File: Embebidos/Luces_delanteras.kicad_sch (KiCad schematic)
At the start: 14 parts, among them J3 Pantallas I2C, J4 Luz_delantera, J5 Joystick, J6 RJ45, J7 RJ45, Q3 BSS138, Q4 DMP3056LSDQ-13

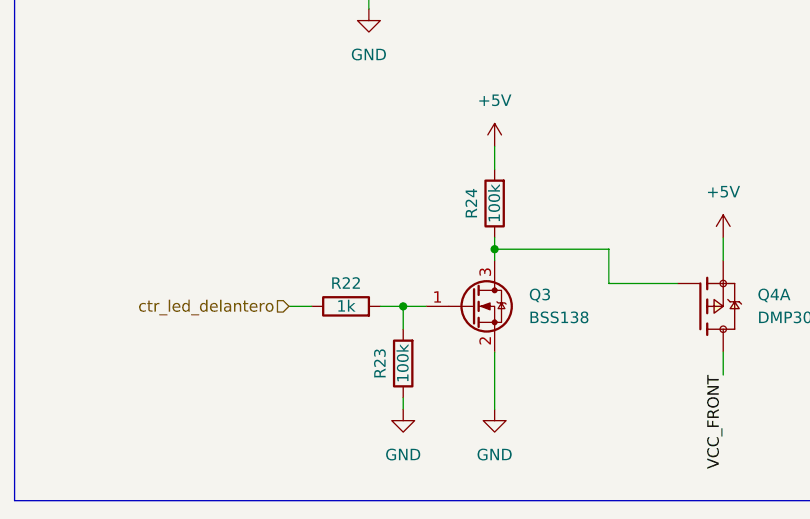
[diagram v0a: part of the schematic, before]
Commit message: nosex2
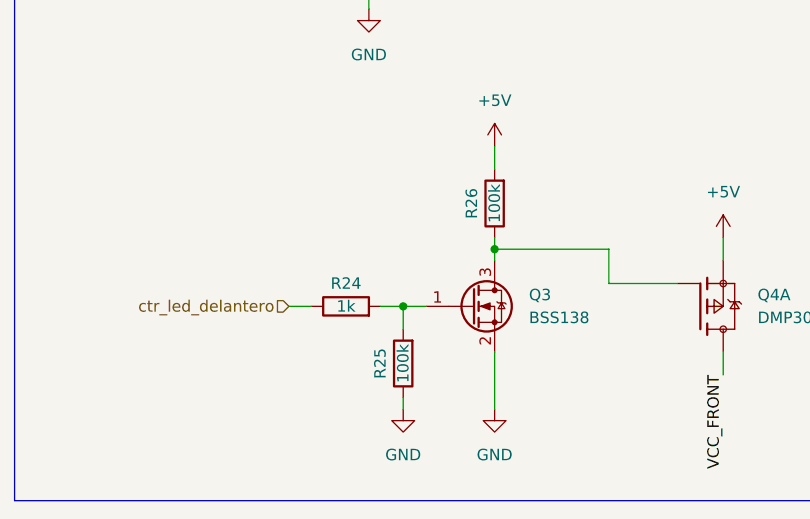
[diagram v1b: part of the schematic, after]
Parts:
- renumbered R22 to R24, R23 to R25, R24 to R26
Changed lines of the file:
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@@
   (symbol (lib_id "Device:R") (at 186.69 143.51 90) (unit 1)
     (in_bom yes) (on_board yes)
-    (property "Reference" "R22" (id 0) (at 186.69 140.97 90))
+    (property "Reference" "R24" (id 0) (at 186.69 140.97 90))
     (property "Value" "1k" (id 1) (at 186.69 143.51 90))
     (property "Footprint" "" (id 2) (at 186.69 145.288 90)
@@
   (symbol (lib_id "Device:R") (at 193.04 149.86 180) (unit 1)
     (in_bom yes) (on_board yes)
-    (property "Reference" "R23" (id 0) (at 190.5 149.86 90))
+    (property "Reference" "R25" (id 0) (at 190.5 149.86 90))
     (property "Value" "100k" (id 1) (at 193.04 149.86 90))
     (property "Footprint" "" (id 2) (at 194.818 149.86 90)
@@
   (symbol (lib_id "Device:R") (at 203.2 132.08 180) (unit 1)
     (in_bom yes) (on_board yes)
-    (property "Reference" "R24" (id 0) (at 200.66 132.08 90))
+    (property "Reference" "R26" (id 0) (at 200.66 132.08 90))
     (property "Value" "100k" (id 1) (at 203.2 132.08 90))
     (property "Footprint" "" (id 2) (at 204.978 132.08 90)

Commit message: r33
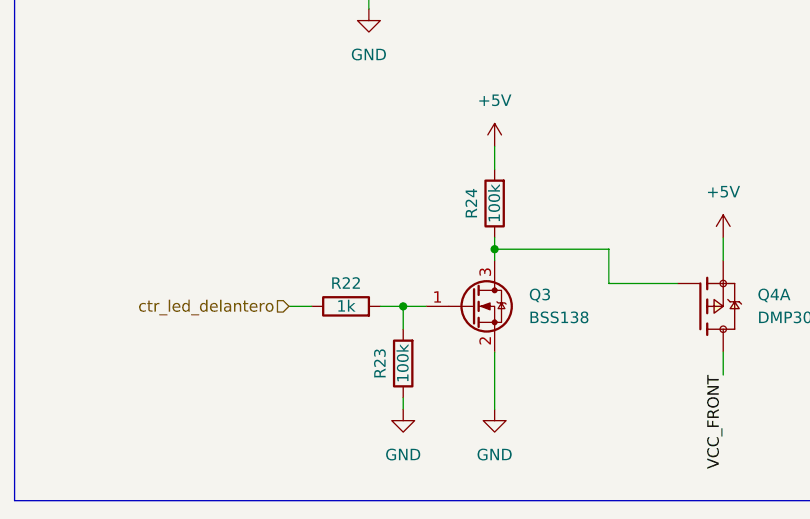
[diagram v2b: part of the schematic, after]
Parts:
- renumbered R24 to R22, R25 to R23, R26 to R24
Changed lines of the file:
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@@
   (symbol (lib_id "Device:R") (at 186.69 143.51 90) (unit 1)
     (in_bom yes) (on_board yes)
-    (property "Reference" "R24" (id 0) (at 186.69 140.97 90))
+    (property "Reference" "R22" (id 0) (at 186.69 140.97 90))
     (property "Value" "1k" (id 1) (at 186.69 143.51 90))
     (property "Footprint" "" (id 2) (at 186.69 145.288 90)
@@
   (symbol (lib_id "Device:R") (at 193.04 149.86 180) (unit 1)
     (in_bom yes) (on_board yes)
-    (property "Reference" "R25" (id 0) (at 190.5 149.86 90))
+    (property "Reference" "R23" (id 0) (at 190.5 149.86 90))
     (property "Value" "100k" (id 1) (at 193.04 149.86 90))
     (property "Footprint" "" (id 2) (at 194.818 149.86 90)
@@
   (symbol (lib_id "Device:R") (at 203.2 132.08 180) (unit 1)
     (in_bom yes) (on_board yes)
-    (property "Reference" "R26" (id 0) (at 200.66 132.08 90))
+    (property "Reference" "R24" (id 0) (at 200.66 132.08 90))
     (property "Value" "100k" (id 1) (at 203.2 132.08 90))
     (property "Footprint" "" (id 2) (at 204.978 132.08 90)
